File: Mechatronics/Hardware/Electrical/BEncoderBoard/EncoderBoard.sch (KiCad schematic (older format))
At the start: 50 parts, among them IC1 RN4020-V_RM120, IC2 TP4056, IC3 DW01+G, J1 Conn_01x07_Male, J2 GNDPWR, J4 Barrel_Jack_Switch, J5 Batt+, J7 Batt-, Q1 FS8205, Q2 Q_PMOS_GSD, Q3 Q_PMOS_GSD, U1 STM32F103C8T6, U2 ITR1802, U3 ITR1802, U4 82402305, U5 SSD1306OLED, U6 LTC3240, Y1 8Mhz

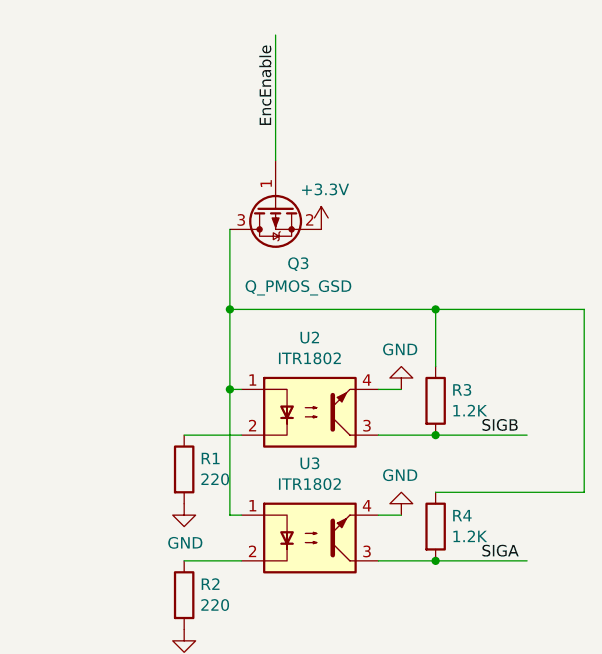
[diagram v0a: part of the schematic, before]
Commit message: Added changes
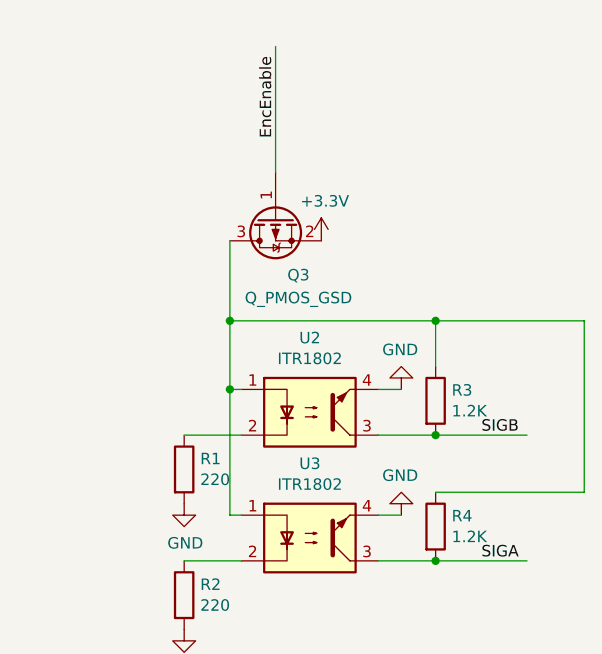
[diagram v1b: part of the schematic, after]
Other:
- moved on the sheet: Q3
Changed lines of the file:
@@
 L Encoder:Q_PMOS_GSD Q3
 U 1 1 5D553268
-P 14400 1550
-F 0 "Q3" H 14500 1350 50  0000 C CNN
-F 1 "Q_PMOS_GSD" H 14500 1250 50  0000 C CNN
-F 2 "Encoder:SOT-23" V 14600 1400 50  0001 C CNN
-F 3 "~" V 14400 1600 50  0001 C CNN
-	1    14400 1550
+P 14400 1600
+F 0 "Q3" H 14500 1400 50  0000 C CNN
+F 1 "Q_PMOS_GSD" H 14500 1300 50  0000 C CNN
+F 2 "Encoder:SOT-23" V 14600 1450 50  0001 C CNN
+F 3 "~" V 14400 1650 50  0001 C CNN
+	1    14400 1600
 	1    0    0    -1
 $EndComp
@@
 Text Label 2100 2650 0    50   ~ 0
 EncEnable
-Text Label 14400 1150 1    50   ~ 0
+Text Label 14400 1200 1    50   ~ 0
 EncEnable
 Wire Wire Line
-	14400 1300 14400 750
+	14400 1350 14400 800
 Wire Wire Line
-	14200 1600 14200 1950
+	14200 1650 14200 2000
 $Comp
 L power:+3.3V #PWR017
 U 1 1 5D59FF5B
-P 14600 1600
-F 0 "#PWR017" H 14600 1450 50  0001 C CNN
-F 1 "+3.3V" H 14615 1773 50  0000 C CNN
-F 2 "" H 14600 1600 50  0001 C CNN
-F 3 "" H 14600 1600 50  0001 C CNN
-	1    14600 1600
+P 14600 1650
+F 0 "#PWR017" H 14600 1500 50  0001 C CNN
+F 1 "+3.3V" H 14615 1823 50  0000 C CNN
+F 2 "" H 14600 1650 50  0001 C CNN
+F 3 "" H 14600 1650 50  0001 C CNN
+	1    14600 1650
 	1    0    0    -1
 $EndComp
 Wire Wire Line
-	15100 2200 15100 1950
+	15100 2200 15100 2000
 Wire Wire Line
-	15100 1950 14200 1950
-Connection ~ 14200 1950
+	15100 2000 14200 2000
+Connection ~ 14200 2000
 Wire Wire Line
-	14200 1950 14200 2300
+	14200 2000 14200 2300
 Wire Wire Line
 	15100 2750 15750 2750
 Wire Wire Line
-	15750 2750 15750 1950
+	15750 2750 15750 2000
 Wire Wire Line
-	15750 1950 15100 1950
-Connection ~ 15100 1950
+	15750 2000 15100 2000
+Connection ~ 15100 2000
 Wire Wire Line
 	6600 6750 7150 6750
